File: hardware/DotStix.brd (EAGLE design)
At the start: 20.3 x 50 mm, 27 parts, among them IC2 SI1145, U1 ATMEGA328P-MU-QFN32, U2 TMP102

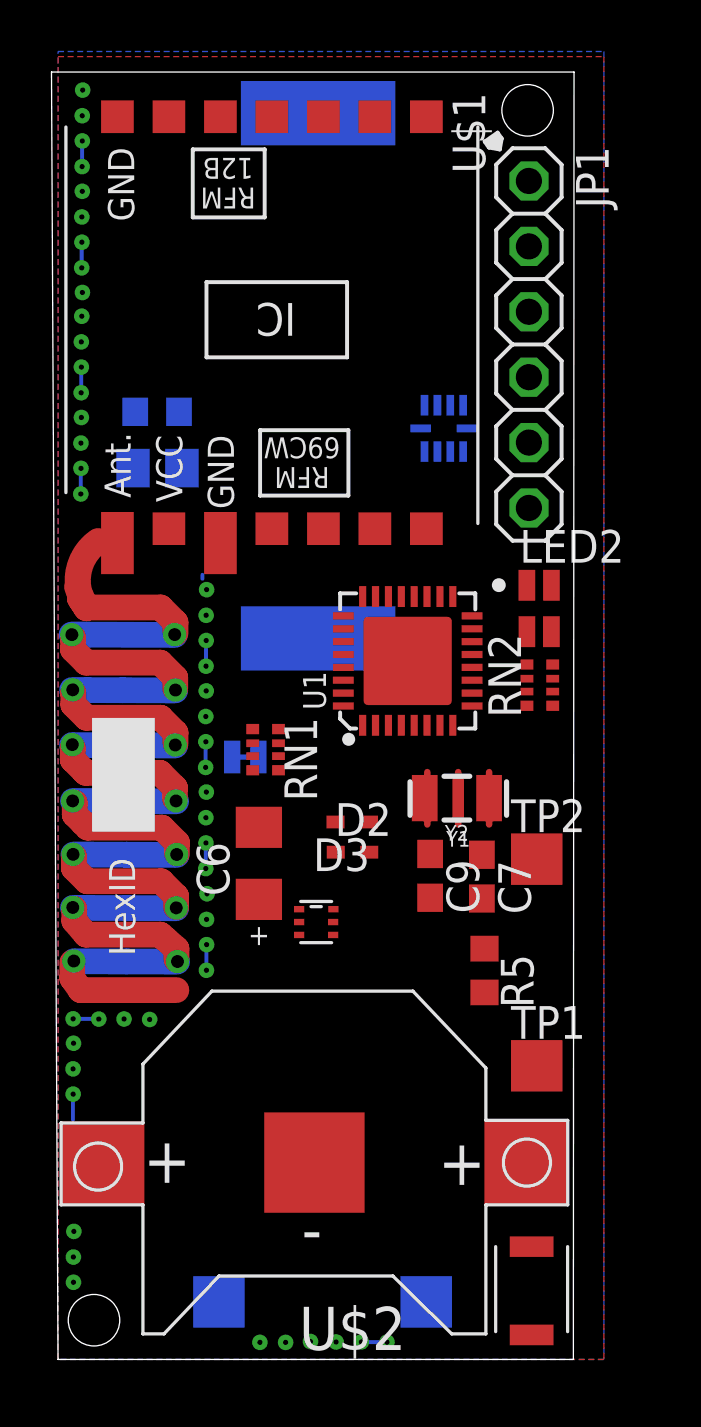
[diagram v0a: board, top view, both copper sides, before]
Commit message: Draft : first routing
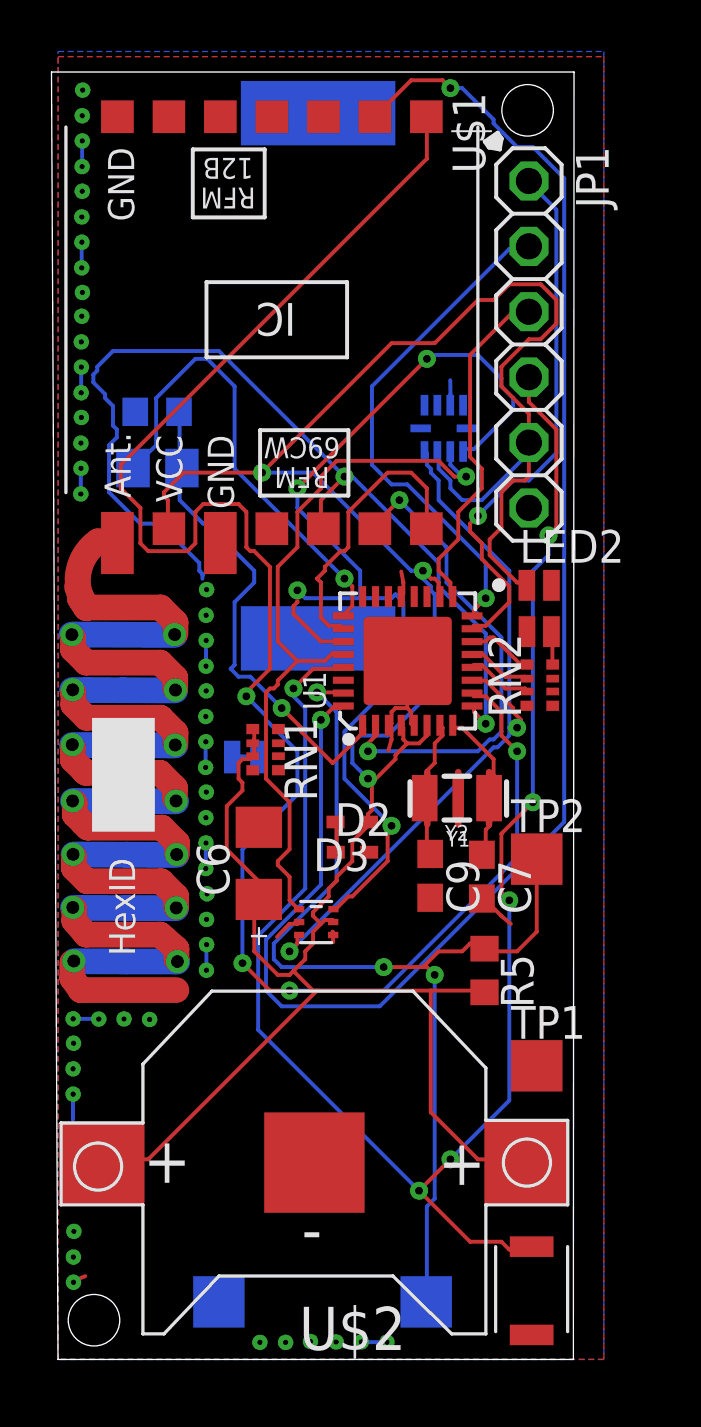
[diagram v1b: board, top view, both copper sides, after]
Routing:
- net +3V3: track 0.00 -> 114.3 mm, vias 0 -> 3
- net RSDO: track 0.00 -> 68.3 mm, vias 0 -> 4
- net RST: track 0.00 -> 65.2 mm, vias 0 -> 6
- net RIRQ: track 0.00 -> 61.9 mm, vias 0 -> 2
- net SDA: track 0.00 -> 42.4 mm, vias 0 -> 4
- net REED: track 0.00 -> 40.1 mm, vias 0 -> 3
- net RSDI: track 0.15 -> 38.1 mm, vias 0 -> 2
- net SCL: track 0.00 -> 28.7 mm, vias 0 -> 1
- net INT_MULTIPLE: track 0.00 -> 28.5 mm, vias 0 -> 2
- net MOSI: track 0.00 -> 21.1 mm, vias 0 -> 1
- net MISO: track 0.00 -> 19.7 mm, vias 0 -> 1
- net LIGHT_SENSE: track 0.00 -> 19.3 mm, vias 0 -> 1
- net RSCK: track 0.00 -> 18.9 mm, vias 0 -> 2
- net LIGHT_SENSE_ENA: track 0.00 -> 18.2 mm, vias 0 -> 1
- net SCK: track 0.00 -> 13.5 mm
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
